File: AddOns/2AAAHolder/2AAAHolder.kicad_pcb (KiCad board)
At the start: 2 copper layers, 47.8 x 50.5 mm, 54 parts, among them P1 Contacts, P2 Contacts, P6 Contacts

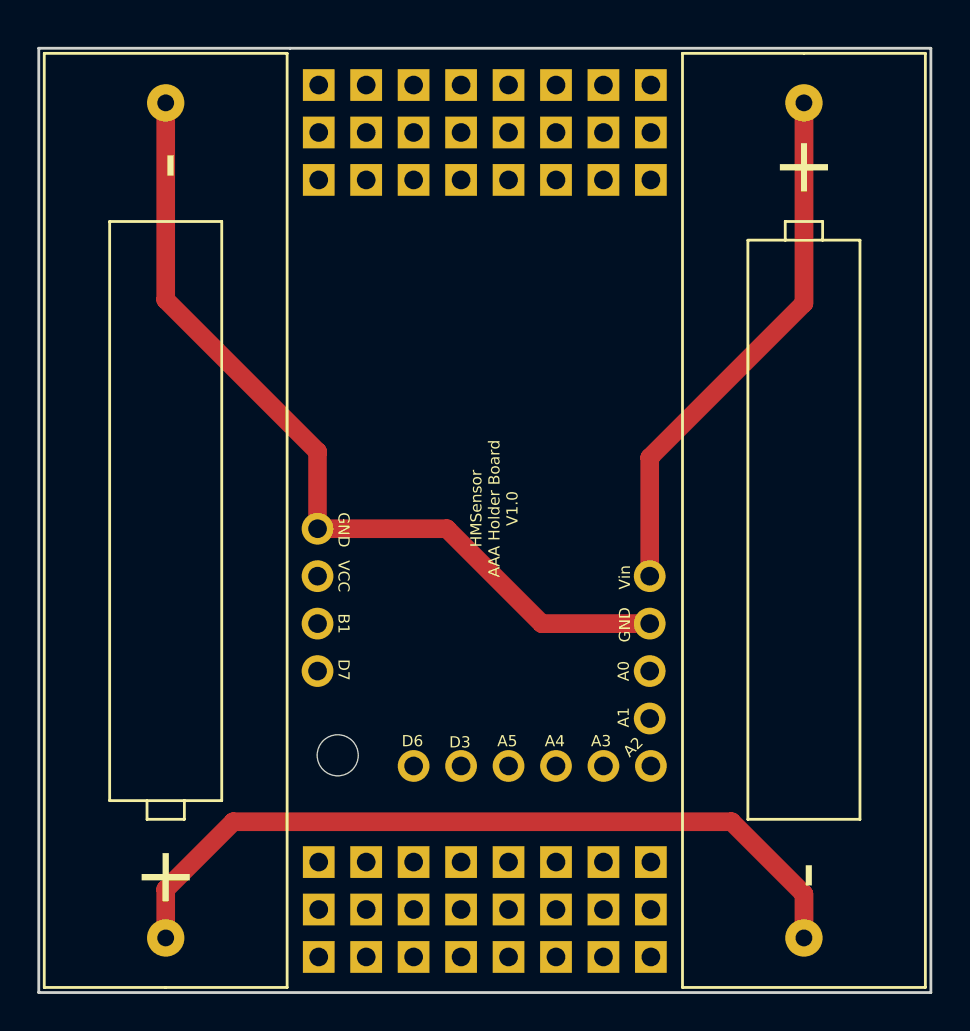
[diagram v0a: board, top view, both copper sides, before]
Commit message: panel added
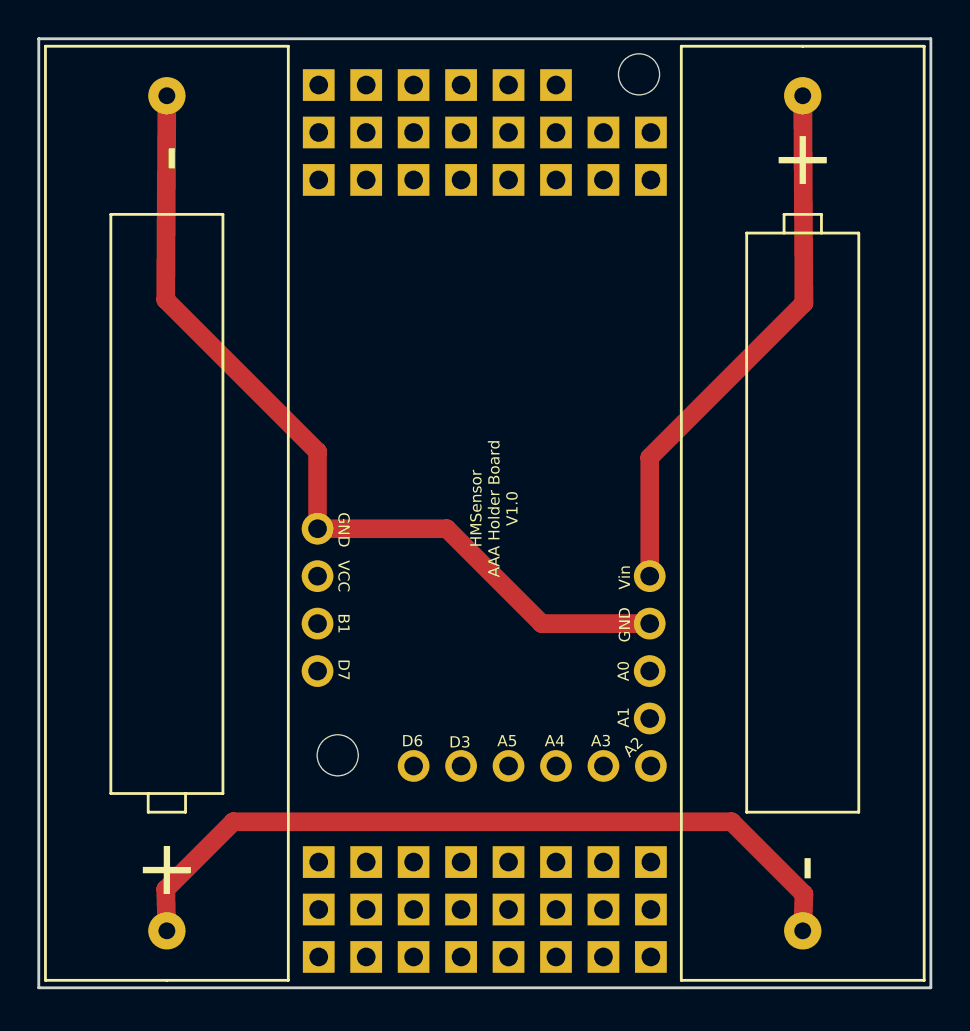
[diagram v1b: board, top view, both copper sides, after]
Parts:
- removed the REF**1 at (188.7, 87.3)
- removed the REF**2 at (186.2, 87.3)
- added REF**: MountingHole_2.2mm_M2, Mounting_Holes:MountingHole_2.2mm_M2, F.Cu at (188.1, 86.7)
- moved REF** 0.39 mm to (196.8, 110.2)
- moved REF** 0.39 mm to (162.8, 110.2)
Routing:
- net (no net): track 42.2 -> 41.5 mm
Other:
- board size 47.8 x 50.5 mm -> 47.8 x 50.8 mm
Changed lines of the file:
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@@
     (links 3)
     (no_connects 0)
-    (area 155.880999 85.268999 203.783001 135.965001)
+    (area 155.880999 84.760999 203.783001 135.711001)
     (thickness 1.6)
-    (drawings 20)
+    (drawings 19)
     (tracks 14)
     (zones 0)
-    (modules 54)
+    (modules 53)
     (nets 14)
   )
@@
     (uvia_drill 0.1)
   )
+  (module Mounting_Holes:MountingHole_2.2mm_M2 (layer F.Cu)
+    (at 188.087 86.741)
+    (descr "Mounting Hole 2.2mm, no annular, M2")
+    (tags "mounting hole 2.2mm no annular m2")
+    (fp_text reference REF** (at -0.127 4.826) (layer F.SilkS) hide
+      (effects (font (size 1 1) (thickness 0.15)))
+    )
+    (fp_text value MountingHole_2.2mm_M2 (at 0 3.2) (layer F.Fab) hide
+      (effects (font (size 1 1) (thickness 0.15)))
+    )
+    (fp_circle (center 0 0) (end 2.2 0) (layer Cmts.User) (width 0.15))
+    (fp_circle (center 0 0) (end 2.45 0) (layer F.CrtYd) (width 0.05))
+    (pad 1 np_thru_hole circle (at 0 0) (size 2.2 2.2) (drill 2.2) (layers *.Cu *.Mask))
+  )
   (module Pin_Headers:Pin_Header_Straight_1x01_Pitch2.54mm (layer F.Cu)
     (at 170.942 92.3925)
@@
     (tags "Through hole pin header THT 1x01 2.54mm single row")
     (fp_text reference REF**3 (at 0 -2.33) (layer F.SilkS) hide
-      (effects (font (size 1 1) (thickness 0.15)))
-    )
-    (fp_text value Pin_Header_Straight_1x01_Pitch2.54mm (at 0 2.33) (layer F.Fab) hide
-      (effects (font (size 1 1) (thickness 0.15)))
-    )
-    (fp_line (start -1.27 -1.27) (end -1.27 1.27) (layer F.Fab) (width 0.1))
-    (fp_line (start -1.27 1.27) (end 1.27 1.27) (layer F.Fab) (width 0.1))
-    (fp_line (start 1.27 1.27) (end 1.27 -1.27) (layer F.Fab) (width 0.1))
-    (fp_line (start 1.27 -1.27) (end -1.27 -1.27) (layer F.Fab) (width 0.1))
-    (fp_line (start -1.8 -1.8) (end -1.8 1.8) (layer F.CrtYd) (width 0.05))
-    (fp_line (start -1.8 1.8) (end 1.8 1.8) (layer F.CrtYd) (width 0.05))
-    (fp_line (start 1.8 1.8) (end 1.8 -1.8) (layer F.CrtYd) (width 0.05))
-    (fp_line (start 1.8 -1.8) (end -1.8 -1.8) (layer F.CrtYd) (width 0.05))
-    (pad 1 thru_hole rect (at 0 0) (size 1.7 1.7) (drill 1) (layers *.Cu *.Mask))
-  )
-  (module Pin_Headers:Pin_Header_Straight_1x01_Pitch2.54mm (layer F.Cu)
-    (at 186.182 87.3125)
-    (descr "Through hole straight pin header, 1x01, 2.54mm pitch, single row")
-    (tags "Through hole pin header THT 1x01 2.54mm single row")
-    (fp_text reference REF**2 (at 0 -2.33) (layer F.SilkS) hide
-      (effects (font (size 1 1) (thickness 0.15)))
-    )
-    (fp_text value Pin_Header_Straight_1x01_Pitch2.54mm (at 0 2.33) (layer F.Fab) hide
-      (effects (font (size 1 1) (thickness 0.15)))
-    )
-    (fp_line (start -1.27 -1.27) (end -1.27 1.27) (layer F.Fab) (width 0.1))
-    (fp_line (start -1.27 1.27) (end 1.27 1.27) (layer F.Fab) (width 0.1))
-    (fp_line (start 1.27 1.27) (end 1.27 -1.27) (layer F.Fab) (width 0.1))
-    (fp_line (start 1.27 -1.27) (end -1.27 -1.27) (layer F.Fab) (width 0.1))
-    (fp_line (start -1.8 -1.8) (end -1.8 1.8) (layer F.CrtYd) (width 0.05))
-    (fp_line (start -1.8 1.8) (end 1.8 1.8) (layer F.CrtYd) (width 0.05))
-    (fp_line (start 1.8 1.8) (end 1.8 -1.8) (layer F.CrtYd) (width 0.05))
-    (fp_line (start 1.8 -1.8) (end -1.8 -1.8) (layer F.CrtYd) (width 0.05))
-    (pad 1 thru_hole rect (at 0 0) (size 1.7 1.7) (drill 1) (layers *.Cu *.Mask))
-  )
-  (module Pin_Headers:Pin_Header_Straight_1x01_Pitch2.54mm (layer F.Cu)
-    (at 188.722 87.3125)
-    (descr "Through hole straight pin header, 1x01, 2.54mm pitch, single row")
-    (tags "Through hole pin header THT 1x01 2.54mm single row")
-    (fp_text reference REF**1 (at 0 -2.33) (layer F.SilkS) hide
       (effects (font (size 1 1) (thickness 0.15)))
     )
@@
   )
   (module Modules:AAA_Holder_Keystone2466 (layer F.Cu)
-    (at 196.9135 110.617)
+    (at 196.85 110.236)
     (fp_text reference REF** (at 0 0 90) (layer F.SilkS) hide
       (effects (font (size 1 1) (thickness 0.15)))
@@
   )
   (module Modules:AAA_Holder_Keystone2466 (layer F.Cu)
-    (at 162.7505 110.617 180)
+    (at 162.814 110.236 180)
     (fp_text reference REF** (at 0 0 270) (layer F.SilkS) hide
       (effects (font (size 1 1) (thickness 0.15)))
@@
     )
   )
-  (gr_line (start 155.956 135.89) (end 155.956 85.344) (angle 90) (layer Edge.Cuts) (width 0.15))
-  (gr_line (start 203.708 135.89) (end 155.956 135.89) (angle 90) (layer Edge.Cuts) (width 0.15))
-  (gr_line (start 203.708 85.344) (end 203.708 135.89) (angle 90) (layer Edge.Cuts) (width 0.15))
-  (gr_line (start 169.418 85.344) (end 203.708 85.344) (angle 90) (layer Edge.Cuts) (width 0.15))
-  (gr_line (start 155.956 85.344) (end 169.418 85.344) (angle 90) (layer Edge.Cuts) (width 0.15))
+  (gr_line (start 155.956 135.636) (end 155.956 84.836) (angle 90) (layer Edge.Cuts) (width 0.15))
+  (gr_line (start 203.708 84.836) (end 203.708 135.636) (angle 90) (layer Edge.Cuts) (width 0.15))
+  (gr_line (start 155.956 84.836) (end 203.708 84.836) (angle 90) (layer Edge.Cuts) (width 0.15))
+  (gr_line (start 155.956 135.636) (end 203.708 135.636) (angle 90) (layer Edge.Cuts) (width 0.15))
   (gr_text D7 (at 172.2755 118.618 270) (layer F.SilkS)
     (effects (font (size 0.6 0.6) (thickness 0.1)))
@@
   )
   (segment (start 193.04 126.746) (end 196.9135 130.6195) (width 1) (layer F.Cu) (net 0))
-  (segment (start 196.9135 130.6195) (end 196.9135 132.967) (width 1) (layer F.Cu) (net 0))
+  (segment (start 196.9135 130.6195) (end 196.85 132.586) (width 1) (layer F.Cu) (net 0) (status 20))
   (segment (start 166.37 126.746) (end 193.04 126.746) (width 1) (layer F.Cu) (net 0))
   (segment (start 162.7505 130.3655) (end 166.37 126.746) (width 1) (layer F.Cu) (net 0))
-  (segment (start 162.7505 132.967) (end 162.7505 130.3655) (width 1) (layer F.Cu) (net 0))
+  (segment (start 162.814 132.586) (end 162.7505 130.3655) (width 1) (layer F.Cu) (net 0) (status 10))
   (segment (start 188.6585 116.1415) (end 182.88 116.1415) (width 1) (layer F.Cu) (net 1))
   (segment (start 170.8785 111.0615) (end 177.8 111.0615) (width 1) (layer F.Cu) (net 1))
   (segment (start 177.8 111.0615) (end 182.88 116.1415) (width 1) (layer F.Cu) (net 1))
   (segment (start 170.8785 111.0615) (end 170.8785 106.934) (width 1) (layer F.Cu) (net 1))
-  (segment (start 162.7505 88.267) (end 162.7505 98.806) (width 1) (layer F.Cu) (net 1))
+  (segment (start 162.814 87.886) (end 162.7505 98.806) (width 1) (layer F.Cu) (net 1) (status 10))
   (segment (start 162.7505 98.806) (end 170.8785 106.934) (width 1) (layer F.Cu) (net 1))
   (segment (start 188.6585 107.2515) (end 196.9135 98.9965) (width 1) (layer F.Cu) (net 10))
-  (segment (start 196.9135 98.9965) (end 196.9135 88.267) (width 1) (layer F.Cu) (net 10))
+  (segment (start 196.9135 98.9965) (end 196.85 87.886) (width 1) (layer F.Cu) (net 10) (status 20))
   (segment (start 188.6585 113.6015) (end 188.6585 107.2515) (width 1) (layer F.Cu) (net 10))
 )
